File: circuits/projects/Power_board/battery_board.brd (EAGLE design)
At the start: 150 x 100 mm, 37 parts

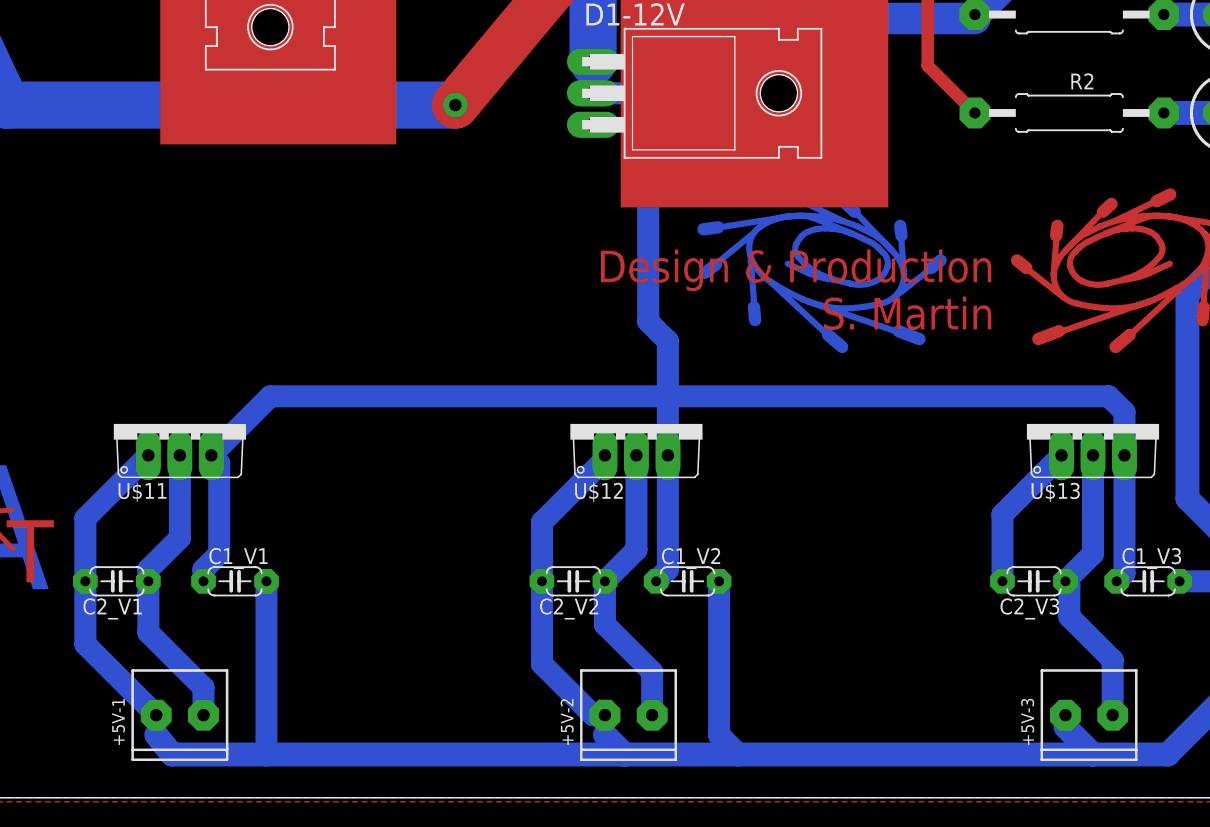
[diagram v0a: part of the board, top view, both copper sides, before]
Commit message: board
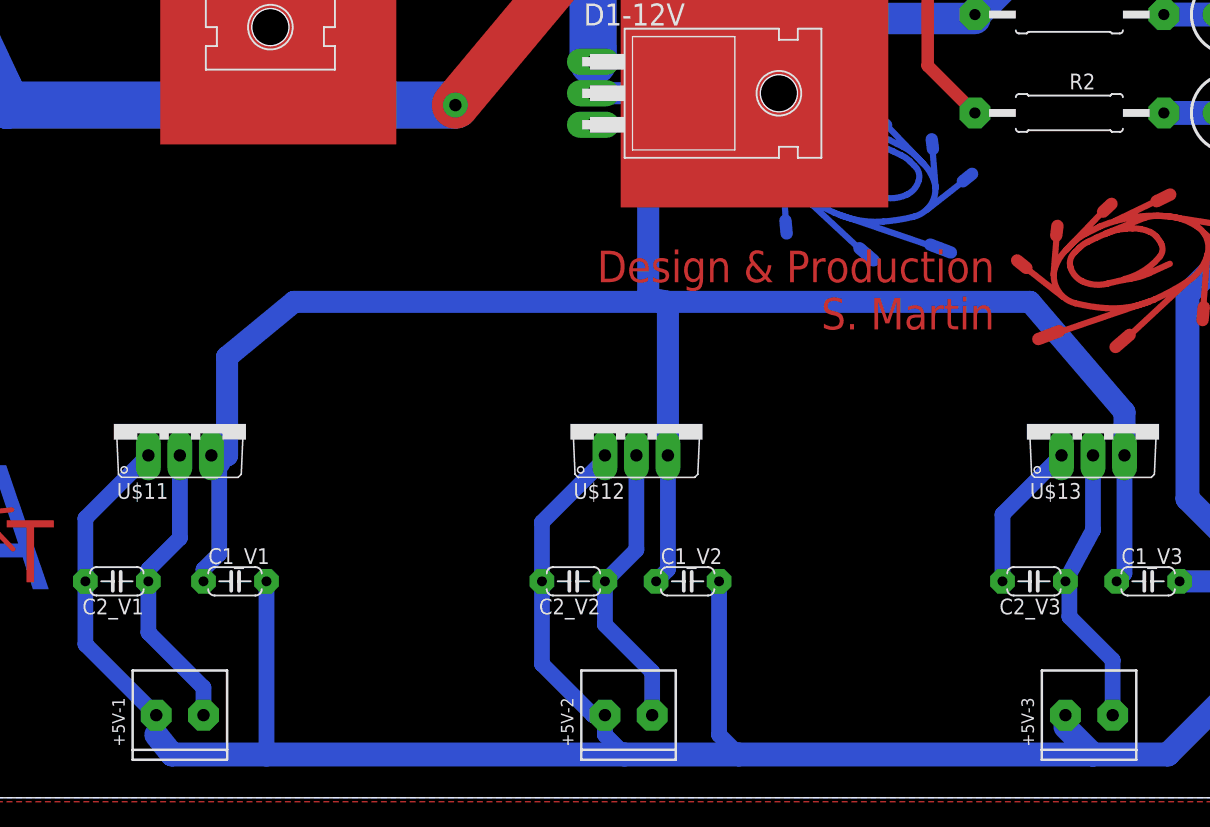
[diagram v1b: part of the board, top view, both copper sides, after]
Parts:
- moved U$8 7.43 mm to (108.0, 50.5)
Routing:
- net 12V: track 239.2 -> 251.0 mm
